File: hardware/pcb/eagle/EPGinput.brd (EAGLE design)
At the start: 78.8 x 22.4 mm, 22 parts, among them J2 54-00248, J3 BNCPTH, U1 ADA4530-1, U2 ADA4530-1, U3 ADA4940-1

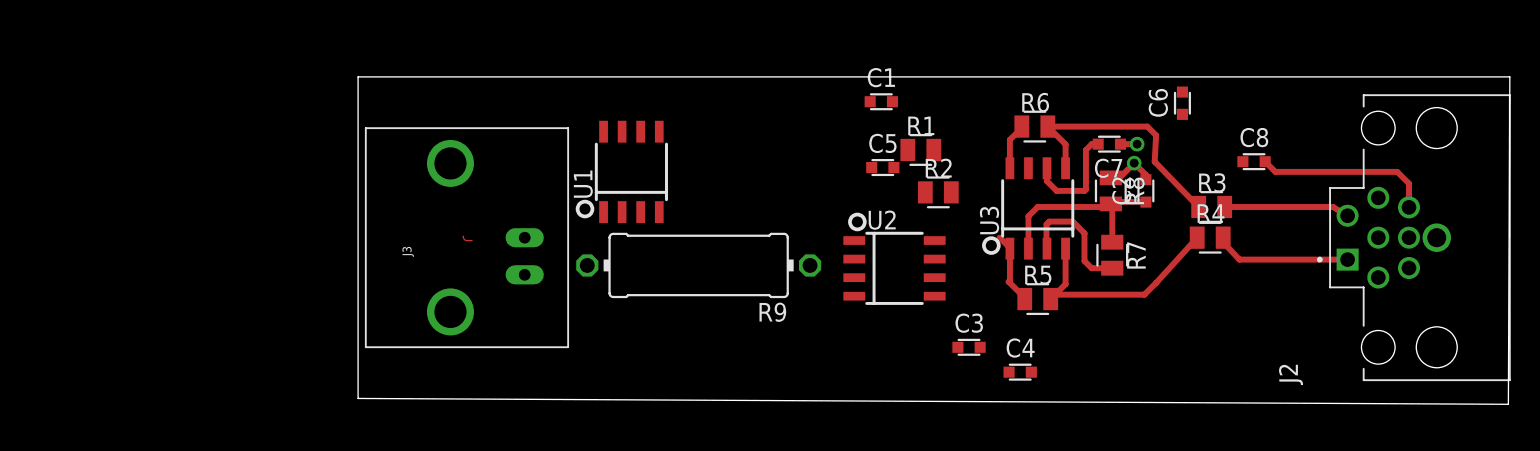
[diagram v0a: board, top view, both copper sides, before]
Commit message: Eagle PCB updates
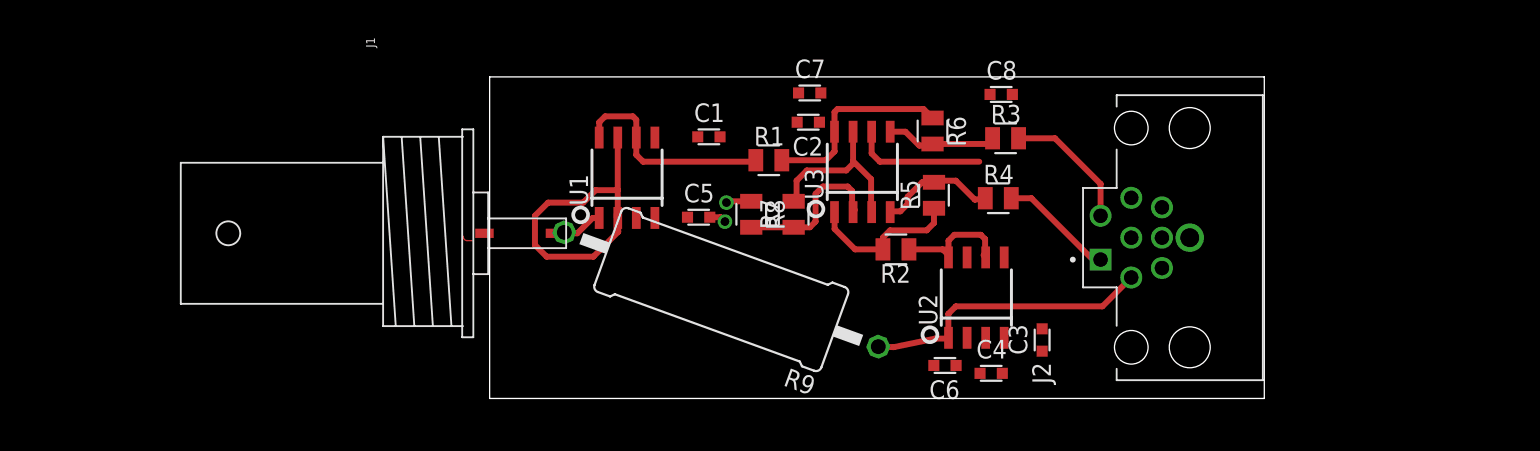
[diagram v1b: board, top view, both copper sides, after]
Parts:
- removed J3: BNCPTH, SparkFun-Connectors:BNC
- added J1: BNCBJ21, STEVES_BU:BNC-BJ21
- R9: device resistor:0414/15 -> resistor:0617/22
- moved R8 24.7 mm to (26.9, 1.60)
- moved C6 24.2 mm to (40.2, -8.74), turned to 180 degrees
- moved C2 23.6 mm to (30.8, 7.90), turned to 180 degrees
- moved R7 22.0 mm to (29.8, 1.60), turned to 90 degrees
- moved C7 20.8 mm to (30.9, 9.90), turned to 0 degrees
- moved C8 17.9 mm to (44.0, 9.80)
- moved J2 16.9 mm to (52.9, 0.00)
- moved R3 14.9 mm to (44.3, 6.80)
- moved R4 14.7 mm to (43.8, 2.70)
- moved C5 13.1 mm to (23.3, 1.40)
- moved U3 12.3 mm to (34.5, 4.50)
- moved C1 12.0 mm to (24.0, 6.90)
- moved R1 10.4 mm to (28.1, 5.30)
- moved R5 10.0 mm to (39.4, 2.90), turned to 90 degrees
- moved R6 7.01 mm to (39.3, 7.30), turned to 270 degrees
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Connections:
- net N$5 renamed SIGOUT
- net N$8 renamed VSOUT
- net GND: now also J1.P$1; no longer J3.GND
- net N$2: now also J1.P$2; no longer J3.S
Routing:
- net N$3: track 0.00 -> 21.9 mm
- net VS: track 0.00 -> 20.1 mm
- net SIGOUT: track 0.00 -> 14.5 mm
- net N$6: track 3.08 -> 13.6 mm
- net N$20: track 17.7 -> 7.99 mm
- net 5V0: track 20.8 -> 12.2 mm
- net VSOUT: track 0.00 -> 8.38 mm
- net N$19: track 15.3 -> 8.23 mm
- net N$7: track 5.08 -> 11.2 mm
- net N$2: track 0.00 -> 3.46 mm
- net N$1: track 13.7 -> 10.7 mm
- net GND: track 5.05 -> 3.10 mm
- net N$10: track 9.74 -> 7.98 mm
- net -5V: track 7.57 -> 9.08 mm
- net N$9: track 8.58 -> 9.09 mm
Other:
- board size 78.8 x 22.4 mm -> 53 x 22 mm

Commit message: board out
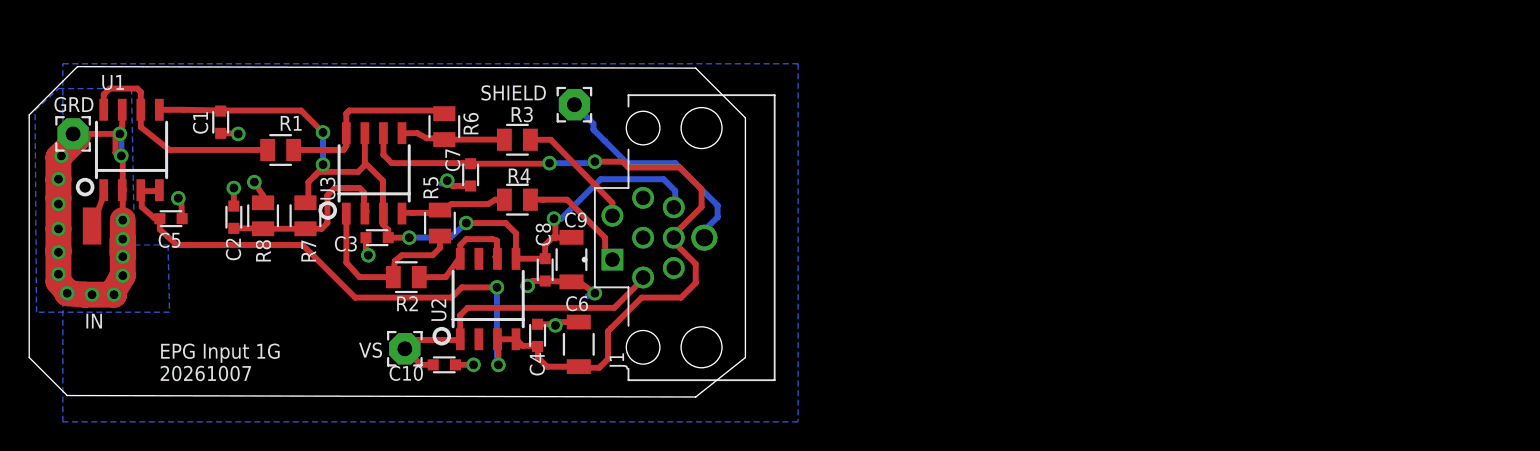
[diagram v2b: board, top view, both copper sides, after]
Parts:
- removed J2: 54-00248, 54-00248:TENSILITY_54-00248
- removed R9: (no value), resistor:0617/22
- added C10: 0.1, STEVES_BU:0603S
- added C9: 10, STEVES_BU:1206S
- added GRD, SHIELD, VS: (no value), wirepad:2,15/1,0
- added IN: (no value), wirepad:SMD1,27-2,54
- added U$1: POMONA2397, STEVES_BU:POMONA2397
- C6: value (none) -> 10; device STEVES_BU:0603S -> STEVES_BU:1206S
- J1: value BNCBJ21 -> 54-00248; device STEVES_BU:BNC-BJ21 -> 54-00248:TENSILITY_54-00248
- moved C3 46.0 mm to (1.30, 0.00), turned to 180 degrees
- moved C2 39.8 mm to (-8.50, 1.40), turned to 90 degrees
- moved C5 36.1 mm to (-12.8, 1.30)
- moved U1 34.0 mm to (-15.5, 6.00)
- moved R5 33.9 mm to (5.60, 1.00)
- moved R2 33.6 mm to (3.30, -2.70)
- moved C8 33.4 mm to (12.8, -2.20), turned to 90 degrees
- moved C1 33.4 mm to (-9.40, 7.90), turned to 270 degrees
- moved R1 33.4 mm to (-5.30, 6.00)
- moved R6 33.4 mm to (5.90, 7.60)
- moved R3 33.4 mm to (10.9, 6.70)
- moved R7 33.4 mm to (-3.60, 1.50)
- moved R8 33.4 mm to (-6.50, 1.50)
- moved U2 33.4 mm to (8.90, -4.20)
- moved U3 33.4 mm to (1.10, 4.40)
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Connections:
- removed net -5V: C7.2, U3.6
- removed net N$2: J1.P$2, R9.2, U1.1
- removed net N$3: U1.2, U1.7
- new net GUARD: GRD.1, U1.2, U1.7
- new net PROBE: IN.1, U1.1
- net -5V0: now also C6.1, C7.2, J1.5, U3.6; no longer J2.5
- net 5V0: now also C9.1, J1.4; no longer J2.4
- net GND: now also C10.2, C6.2, C9.2, J1.6; no longer J1.P$1, J2.6
- net N$10: now also J1.1; no longer J2.1
- net N$9: now also J1.2; no longer J2.2
- net SHIELD: now also J1.8, J1.S1, SHIELD.1; no longer J2.8, J2.S1
- net VS: now also C10.1, J1.7, VS.1; no longer J2.7, R9.1
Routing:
- net -5V0: track 0.00 -> 87.3 mm, vias 0 -> 4
- net GUARD: track 0.00 -> 74.8 mm, vias 0 -> 15
- net 5V0: track 12.2 -> 57.8 mm, vias 0 -> 5
- net N$3: track 21.9 -> 0.00 mm
- net GND: track 3.10 -> 20.4 mm, vias 2 -> 10
- net SHIELD: track 0.00 -> 15.5 mm
- net -5V: track 9.08 -> 0.00 mm
- net N$2: track 3.46 -> 0.00 mm
- net PROBE: track 0.00 -> 2.59 mm
- net N$7: track 11.2 -> 13.4 mm
- net N$1: track 10.7 -> 12.7 mm
- net VS: track 20.1 -> 21.6 mm
- net SIGOUT: track 14.5 -> 15.6 mm
- net N$6: track 13.6 -> 12.8 mm
- net N$19: track 8.23 -> 7.43 mm
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- added copper zone on layer 16, net GND
- added copper zone on layer 16, net GUARD
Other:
- board size 53 x 22 mm -> 49 x 22.6 mm
- board text added: "EPG Input 1G 20261007"
